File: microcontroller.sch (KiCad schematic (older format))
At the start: 34 parts, among them SW1 SW_Push, U1 74HC595, U2 74HC595, U3 ESP32-WROOM, U4 74HC595, U5 74HC595

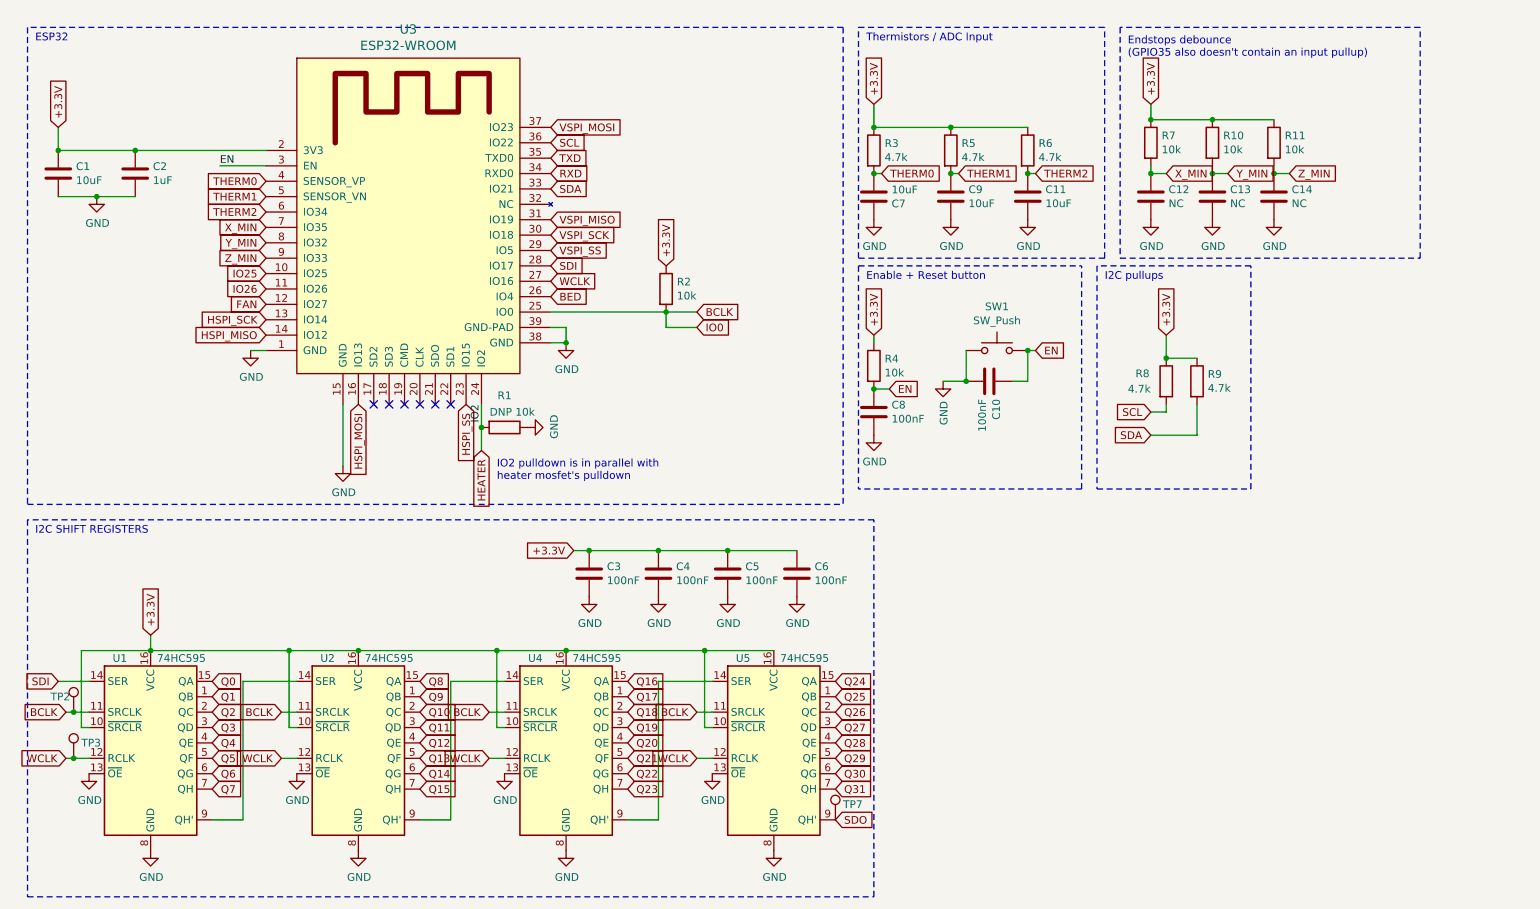
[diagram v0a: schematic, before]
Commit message: Prototype R3
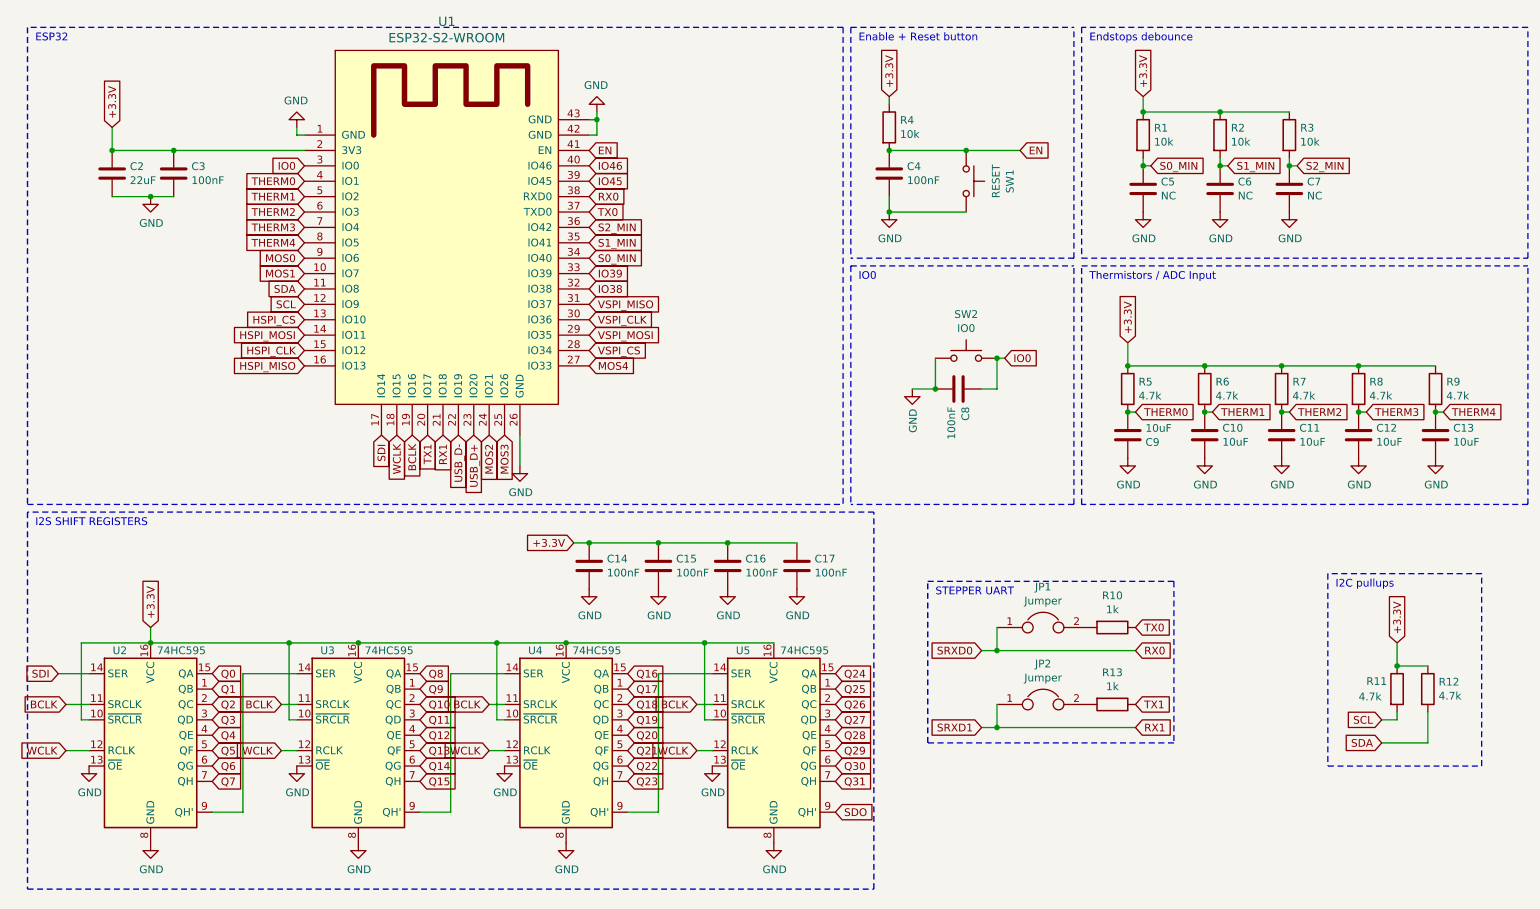
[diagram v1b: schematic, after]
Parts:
- removed C1: 10uF, Capacitor_SMD:C_0805_2012Metric, symbol esp32controller-rescue:C-Device
- removed C10: 100nF, Capacitor_SMD:C_0603_1608Metric, symbol Device:C
- removed R1: DNP 10k, Resistor_SMD:R_0603_1608Metric, symbol Device:R
- removed R2: 10k, Resistor_SMD:R_0603_1608Metric, symbol Device:R
- removed TP2, TP3, TP7: TestPoint, TestPoint:TestPoint_Pad_D1.5mm, symbol Connector:TestPoint
- removed U3: ESP32-WROOM, ESP32-footprints-Lib:ESP32-WROOM, symbol esp32controller-rescue:ESP32-WROOM-ESP32-footprints-Shem-Lib
- added C12, C13: 10uF, Capacitor_SMD:C_0805_2012Metric, symbol Device:C
- added C3: 100nF, Capacitor_SMD:C_0603_1608Metric, symbol esp32controller-rescue:C-Device
- added C8: 100nF, Capacitor_SMD:C_0603_1608Metric, symbol Device:C
- added JP1, JP2: Jumper, Connector_PinHeader_2.54mm:PinHeader_1x02_P2.54mm_Vertical, symbol Device:Jumper
- added R10, R13: 1k, Resistor_SMD:R_0603_1608Metric, symbol Device:R
- added R8, R9: 4.7k, Resistor_SMD:R_0603_1608Metric, symbol Device:R
- added SW2: IO0, Button_Switch_SMD:SW_Push_1P1T_NO_6x6mm_H9.5mm, symbol Switch:SW_Push
- added U1: ESP32-S2-WROOM, ESP32Controller:esp32-s2-wrooom, symbol ESP32Controller:ESP32-S2-WROOM
- C2: value 1uF -> 22uF; footprint Capacitor_SMD:C_0603_1608Metric -> Capacitor_SMD:C_0805_2012Metric
- SW1: value SW_Push -> RESET
- renumbered C9 to C10, C3 to C14, C4 to C15, C5 to C16, C6 to C17, C8 to C4, C12 to C5, C13 to C6, C14 to C7, C7 to C9, R7 to R1, R8 to R11, R9 to R12, R10 to R2, R11 to R3, R3 to R5, R5 to R6, R6 to R7, U1 to U2, U2 to U3
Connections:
- net +3.3V: now also C3.1, R8.1, R9.1, U1.2 (3V3)
- net BCLK: now also U1.19 (IO16)
- net EN: now also SW1.1, U1.41 (EN); no longer SW1.2
- net GND: now also SW1.2, C12.2, C13.2, C3.2, C8.2, SW2.1, U1.1 (GND), U1.26 (GND), U1.42 (GND), U1.43 (GND); no longer SW1.1
- net HSPI_MISO: now also U1.16 (IO13)
- net HSPI_MOSI: now also U1.14 (IO11)
- net SCL: now also U1.12 (IO9)
- net SDA: now also U1.11 (IO8)
- net SDI: now also U1.17 (IO14)
- net THERM0: now also U1.4 (IO1)
- net THERM1: now also U1.5 (IO2)
- net THERM2: now also U1.6 (IO3)
- net VSPI_MISO: now also U1.31 (IO37)
- net VSPI_MOSI: now also U1.29 (IO35)
- net WCLK: now also U1.18 (IO15)
- net X_MIN renamed S0_MIN
- net S0_MIN: now also U1.34 (IO40)
- net Y_MIN renamed S1_MIN
- net S1_MIN: now also U1.35 (IO41)
- net Z_MIN renamed S2_MIN
- net S2_MIN: now also U1.36 (IO42)
- new net: JP1.2, R10.2
- new net: JP2.2, R13.2
- new net HSPI_CLK: U1.15 (IO12)
- new net HSPI_CS: U1.13 (IO10)
- new net IO0: C8.1, SW2.2, U1.3 (IO0)
- new net IO38: U1.32 (IO38)
- new net IO39: U1.33 (IO39)
- new net IO45: U1.39 (IO45)
- new net IO46: U1.40 (IO46)
- new net MOS0: U1.9 (IO6)
- new net MOS1: U1.10 (IO7)
- new net MOS2: U1.24 (IO21)
- new net MOS3: U1.25 (IO26)
- new net MOS4: U1.27 (IO33)
- new net RX0: JP1.1, U1.38 (RXD0)
- new net RX1: JP2.1, U1.21 (IO18)
- new net THERM3: C12.1, R8.2, U1.7 (IO4)
- new net THERM4: C13.1, R9.2, U1.8 (IO5)
- new net TX0: R10.1, U1.37 (TXD0)
- new net TX1: R13.1, U1.20 (IO17)
- new net USB_D+: U1.23 (IO20)
- new net USB_D-: U1.22 (IO19)
- new net VSPI_CLK: U1.30 (IO36)
- new net VSPI_CS: U1.28 (IO34)
- no-connect marks 6 -> 0
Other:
- note added: "Endstops debounce"
- note added: "I2S SHIFT REGISTERS"
- note added: "IO0"
- note added: "STEPPER UART"
- note removed: "Endstops debounce\n(GPIO35 also doesn't contain an input pullup)"
- note removed: "I2C SHIFT REGISTERS"
- note removed: "IO2 pulldown is in parallel with\nheater mosfet's pulldown"
- moved on the sheet: C10, C11, C14, C15, C16, C17, C4, C5, C6, C7, C9, R1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
